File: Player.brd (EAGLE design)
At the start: 60.9 x 42.5 mm, 60 parts, among them CN1 STEREO-3.5-MJ8435, CON1 UART-S, CON2 MICROSD-DM3, CON3 MINI-USB-, CON4 MOLEX-5251-02-S_LONG, IC1 R5F5631-48LFQFP, IC2 AK4386, IC3 BH3544F, IC4 XC6802A42XMR, IC6 AQM1248-RN, SW1 PUSHSW, SW2 PUSHSW, SW3 PUSHSW, SW4 PUSHSW, SW5 PUSHSW, SW6 PUSHSW, SW7 SLIDESW, X1 6.144MHz

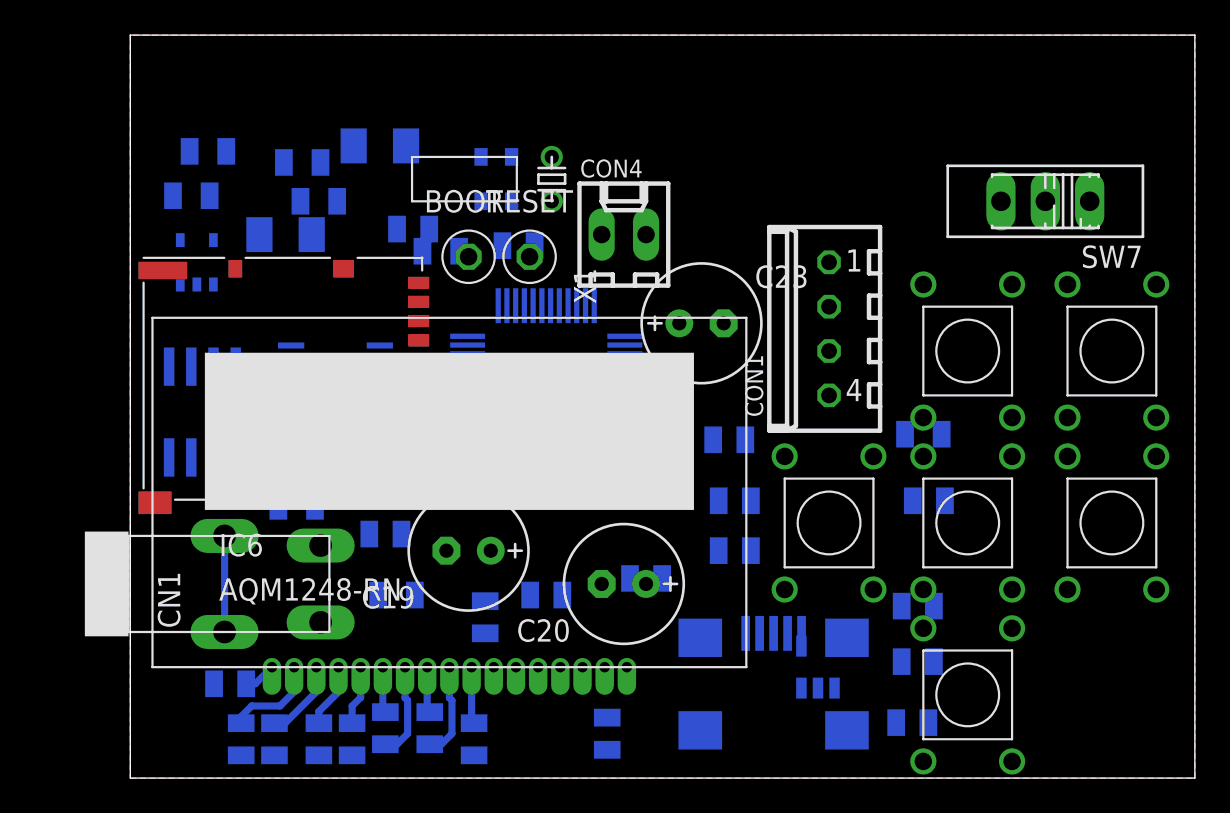
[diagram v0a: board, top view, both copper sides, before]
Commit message: Halfway through wiring
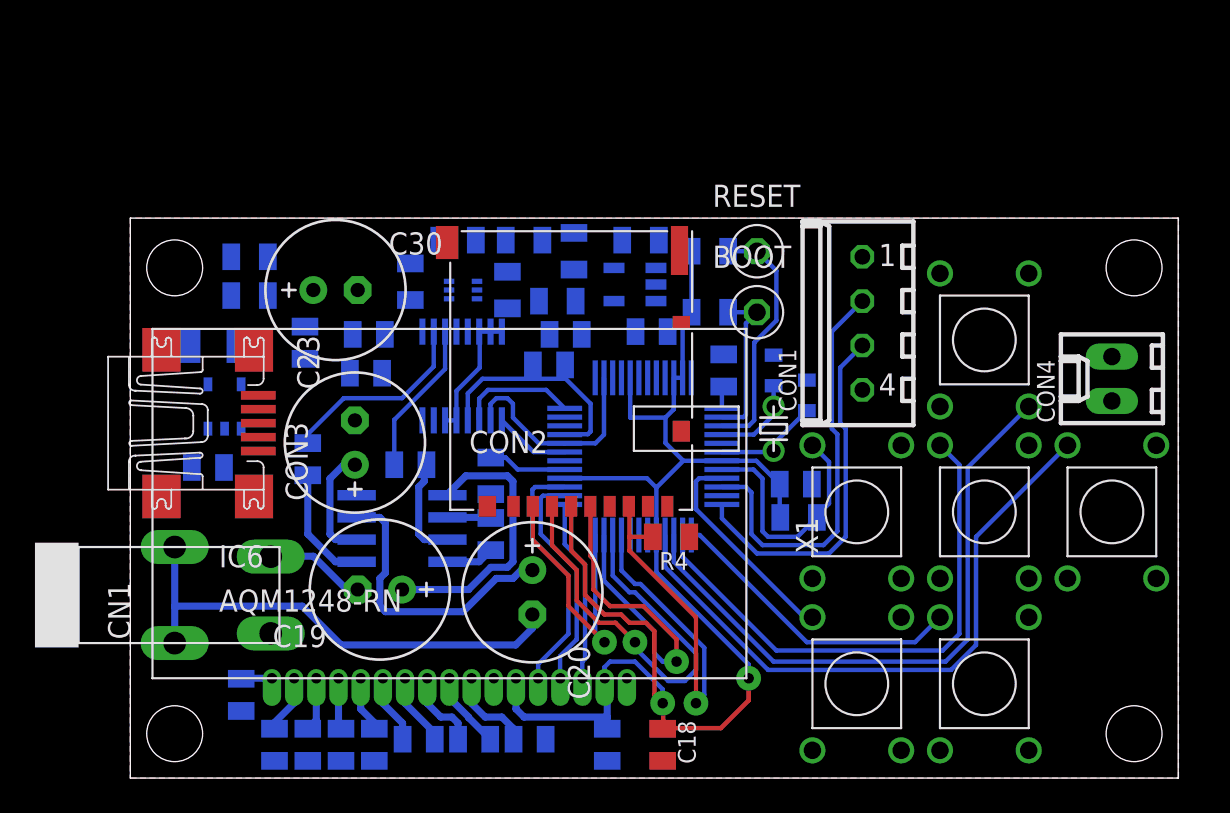
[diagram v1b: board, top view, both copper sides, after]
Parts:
- removed C15: 0.1u, Passive_Robotech:2012-C
- removed D1: RB160M-30TR, Diode_Robotech:D3216
- removed SW7: SLIDESW, Passive_Robotech:SLIDESW
- added C30: 22u, Passive_Robotech:E2,5-8
- added Q1: SSM6L35FE, Transistor_Robotech:2-2N1D
- added R10, R11: 100, Passive_Robotech:2012-R
- added R12: 10k, Passive_Robotech:2012-R
- added R13, R14: 22k, Passive_Robotech:2012-R
- C19, C20, C23: device Passive_Robotech:E2,5-7 -> Passive_Robotech:E2,5-8
- moved C21 39.5 mm to (10.0, 24.9), turned to 270 degrees
- moved CON3 34.8 mm to (5.08, 20.3), flipped to the top, turned to 0 degrees
- moved R4 34.5 mm to (31.0, 13.8), flipped to the top, turned to 180 degrees
- moved C22 34.3 mm to (13.5, 23.2), turned to 180 degrees
- moved CON4 29.1 mm to (56.2, 22.9), turned to 90 degrees
- moved C12 28.5 mm to (38.1, 16.8), turned to 180 degrees
- moved R2 27.8 mm to (33.2, 30.2), turned to 180 degrees
- moved C28 25.2 mm to (20.6, 14.0), turned to 270 degrees
- moved R8 24.9 mm to (20.6, 17.3), turned to 270 degrees
- moved IC4 24.3 mm to (28.9, 28.3), turned to 270 degrees
- moved R1 24.3 mm to (33.2, 26.7), turned to 180 degrees
- moved C24 24.2 mm to (10.2, 18.3), turned to 90 degrees
- moved R3 23.4 mm to (38.3, 14.9), turned to 180 degrees
- moved C14 22.4 mm to (38.7, 21.9), turned to 90 degrees
- moved R6 22.1 mm to (25.4, 30.2), turned to 270 degrees
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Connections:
- new net N$55: IC1.P$40, R13.2, R14.2
- net +3V3: now also IC1.P$17; no longer C22.1, IC3.8
- net +5V: now also C22.1, C26.1, C30.+, IC3.8, Q1.4, R12.1, R13.1, U$1.1, U$1.3; no longer D1.K, SW7.1
- net GND: now also C30.-, Q1.1, R14.1; no longer C15.2
- net N$18: now also IC1.P$37, R10.2; no longer C15.1, IC1.P$17
- net N$19: now also Q1.2, R10.1; no longer CON3.2, IC1.P$18
- net N$21: now also Q1.5, R11.1, R12.2; no longer CON3.3, IC1.P$19
- net N$47: now also Q1.6, R11.2; no longer C26.1, SW7.2, U$1.1, U$1.3
- net N$50: now also Q1.3; no longer D1.A
- net N$54: now also IC1.P$29; no longer IC1.P$37
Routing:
- net +3V3: track 0.00 -> 92.5 mm, vias 0 -> 2
- net N$25: track 0.00 -> 36.3 mm
- net N$26: track 0.00 -> 36.0 mm
- net N$27: track 0.00 -> 31.0 mm
- net N$23: track 0.00 -> 26.2 mm, vias 0 -> 1
- net N$29: track 0.00 -> 25.1 mm, vias 0 -> 1
- net N$13: track 0.00 -> 23.7 mm
- net N$41: track 5.50 -> 28.1 mm
- net N$16: track 0.00 -> 21.5 mm, vias 0 -> 1
- net N$12: track 0.00 -> 20.7 mm
- net N$28: track 0.00 -> 17.4 mm
- net N$37: track 0.00 -> 16.5 mm
- net N$39: track 0.00 -> 16.0 mm
- net N$30: track 0.00 -> 15.8 mm, vias 0 -> 1
- net N$20: track 0.00 -> 14.3 mm
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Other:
- board size 60.9 x 42.5 mm -> 60 x 32.1 mm
